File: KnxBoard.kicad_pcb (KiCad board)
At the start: 2 copper layers, 41 parts, among them IC1 STM32G491KEU6, IC2 NCN5130MNTWG, J1 Conn_01x02, J2 Conn_02x03_Counter_Clockwise, J3 Conn_01x10, J4 Conn_01x10, SW1 SW_Push, Y1 16MHz

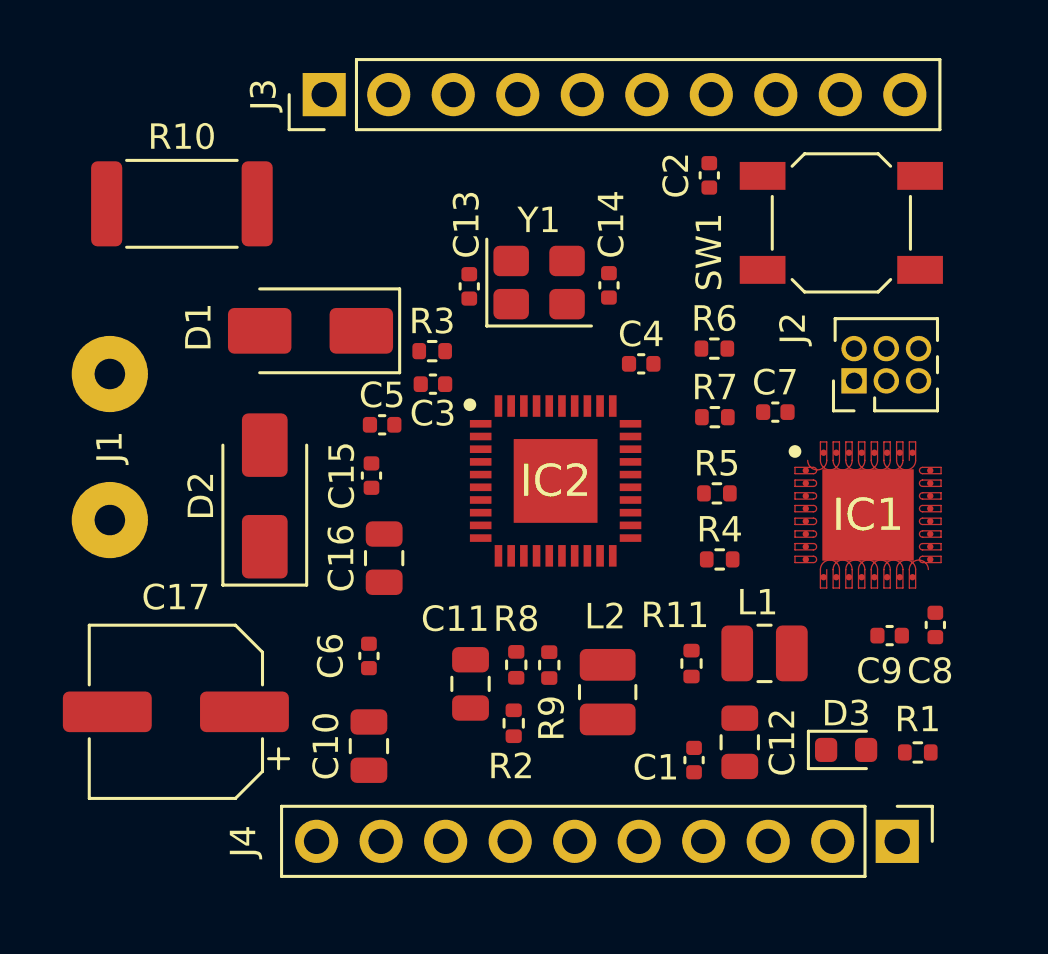
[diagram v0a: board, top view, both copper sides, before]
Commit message: Route
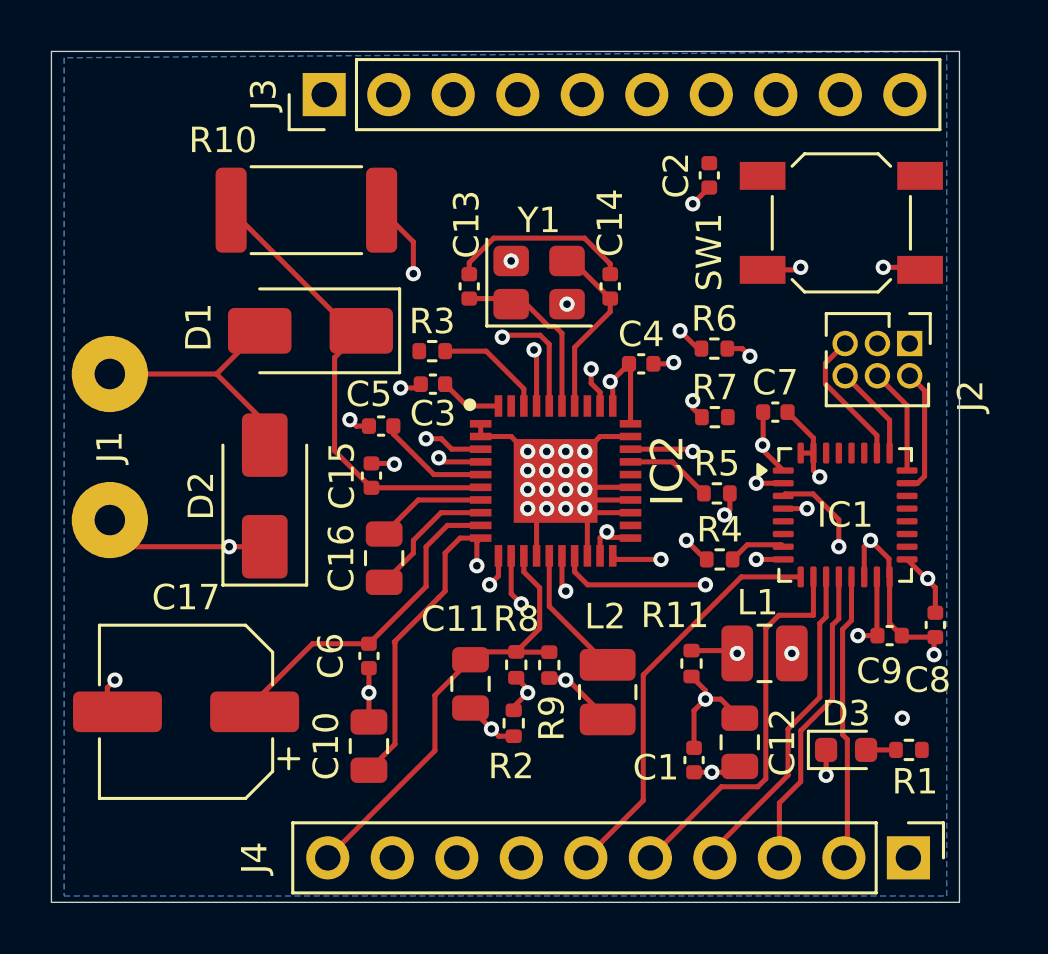
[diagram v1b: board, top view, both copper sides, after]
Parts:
- IC1: footprint Library:QFN50P500X500X60-33N-D -> Package_DFN_QFN:UQFN-32_5x5mm_P0.5mm
- moved R10 4.91 mm to (131.0, 132.2)
- moved J2 2.64 mm to (154.8, 137.5), turned to -90 degrees
- moved IC1 0.90 mm to (152.2, 144.2)
- moved J4 0.78 mm to (154.7, 157.8)
- moved C17 0.40 mm to (126.3, 152.0)
- moved R1 0.36 mm to (154.8, 153.5)
- moved C5 0.06 mm to (134.0, 140.8), turned to 180 degrees
- moved C14 0.06 mm to (143.0, 135.2), turned to 90 degrees
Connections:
- J2 pad 2: Net-(IC1-DEBUG_TX) -> Net-(IC1-SYS_JTMS-SWDIO)
- J2 pad 3: Net-(IC1-DEBUG_RX) -> unconnected-(J2-Pin_3-Pad3)
- J2 pad 5: Net-(IC1-SYS_JTMS-SWDIO) -> Net-(IC1-DEBUG_TX)
- J2 pad 6: unconnected-(J2-Pin_6-Pad6) -> Net-(IC1-DEBUG_RX)
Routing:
- net 3V3: track 0.00 -> 62.7 mm, vias 0 -> 6
- net GND: track 0.00 -> 55.6 mm, vias 0 -> 33
- net Net-(IC1-RCC_OSC_IN): track 0.00 -> 32.8 mm, vias 0 -> 2
- net Net-(IC1-PG10-NRST): track 0.00 -> 29.3 mm, vias 0 -> 2
- net Net-(D1-K): track 0.00 -> 18.6 mm
- net Net-(IC2-V20V): track 0.00 -> 18.0 mm, vias 0 -> 2
- net 12V: track 0.00 -> 17.8 mm
- net Net-(IC2-SAVEB): track 0.00 -> 16.5 mm, vias 0 -> 2
- net Net-(IC1-PA4): track 0.00 -> 15.9 mm
- net Net-(IC1-PA5): track 0.00 -> 15.4 mm
- net Net-(IC2-VFILT): track 0.00 -> 13.3 mm
- net Net-(IC1-PA6): track 0.00 -> 12.9 mm
- net Net-(IC2-TXO): track 0.00 -> 12.0 mm, vias 0 -> 2
- net Net-(IC1-PA7): track 0.00 -> 12.0 mm
- net Net-(IC1-KNX_PROG_LED): track 0.00 -> 11.5 mm, vias 0 -> 2
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- added copper zone on B.Cu, net GND
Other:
- board outline added: 35.8 x 33.5 mm
- copper layers 2 -> 4
- board text added: "KEEP-OUT ZONE"
- board text added: "No F.Cu tracks"
